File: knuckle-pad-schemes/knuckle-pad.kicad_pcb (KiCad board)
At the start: 2 copper layers, 127.6 x 115.3 mm, 67 parts, among them SW1 SW_Push, SW10 SW_Push, SW11 SW_Push, SW12 SW_Push, SW13 SW_Push, SW14 SW_Push, SW15 SW_Push, SW16 SW_Push, SW17 SW_Push, SW18 SW_Push, SW19 SW_Push, SW2 SW_Push, SW20 SW_Push, SW21 SW_Push, SW22 SW_Push, SW23 SW_Push, SW24 SW_Push, SW25 SW_Push, SW26 SW_Push, SW27 SW_Push, SW28 SW_Push, SW29 SW_Push, SW3 SW_Push, SW4 SW_Push, SW5 SW_Push, SW6 SW_Push, SW7 SW_Push, SW8 SW_Push, SW9 SW_Push, U1 ProMicro

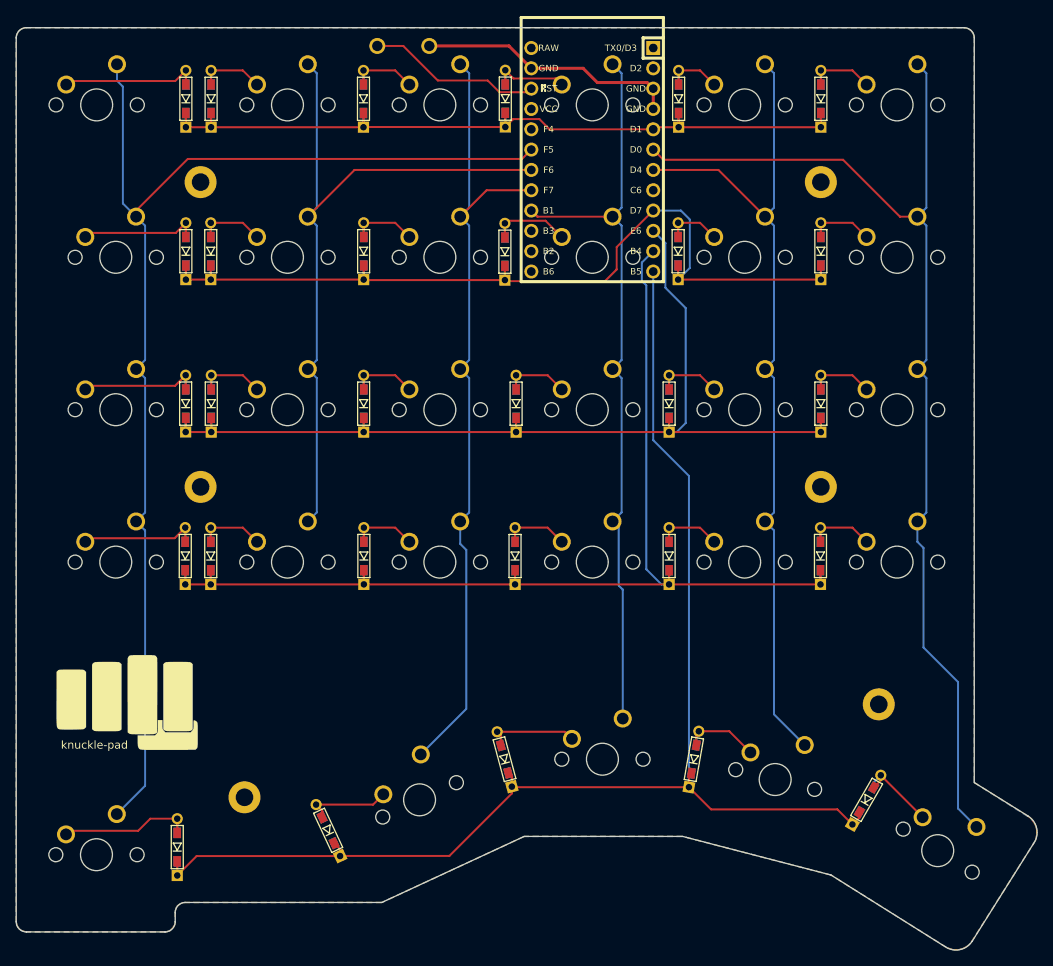
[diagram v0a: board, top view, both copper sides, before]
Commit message: clean up
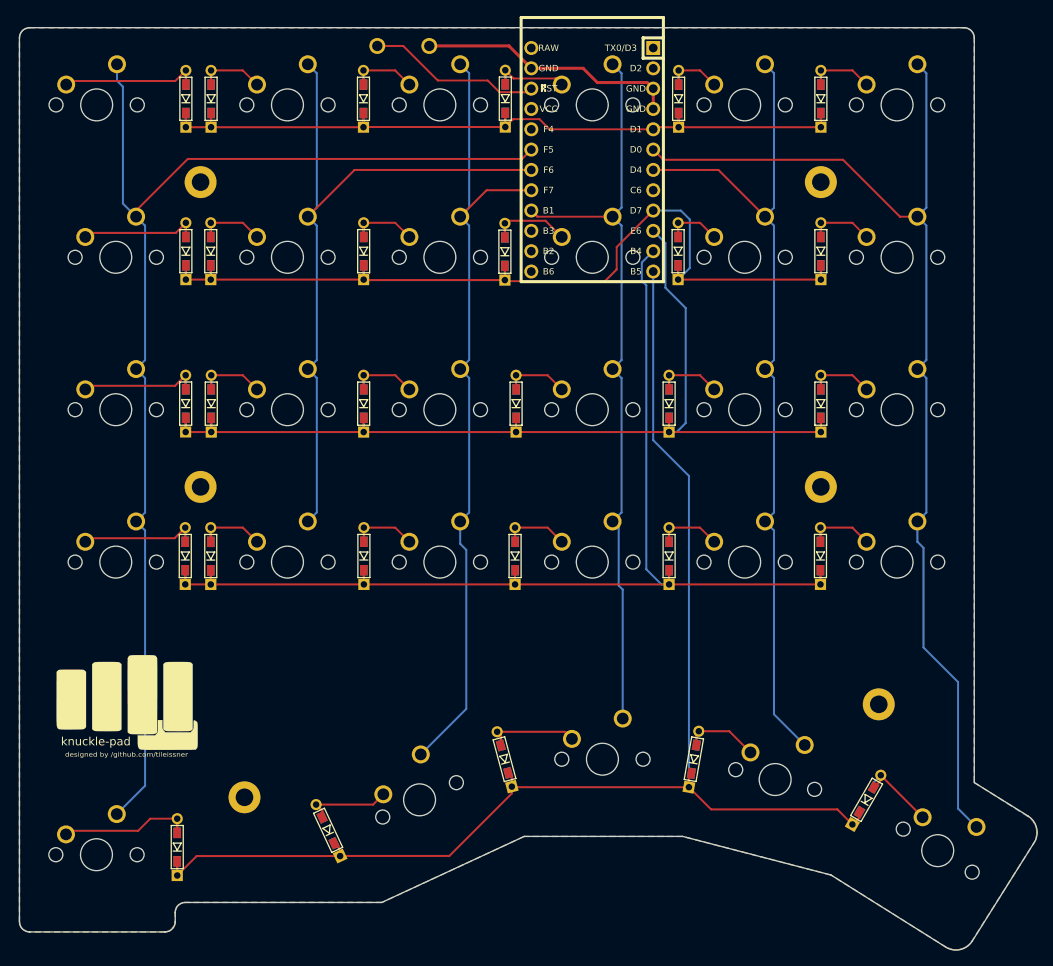
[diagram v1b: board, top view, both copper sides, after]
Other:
- board size 127.6 x 115.3 mm -> 127.2 x 115.3 mm
- board text added: "designed by /github.com/tileissner"
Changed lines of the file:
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@@
   (general
     (thickness 1.6)
-    (drawings 22)
+    (drawings 23)
     (tracks 372)
     (zones 0)
@@
     )
   )
-  (gr_text knuckle-pad (at 90.678 123.444) (layer F.SilkS)
-    (effects (font (size 1 1) (thickness 0.15)))
+  (gr_text "designed by /github.com/tileissner" (at 94.6912 124.64034) (layer F.SilkS)
+    (effects (font (size 0.5842 0.6477) (thickness 0.0762)))
+  )
+  (gr_arc (start 82.5754 35.052) (end 82.5754 33.782) (angle -90) (layer Edge.Cuts) (width 0.05))
+  (gr_arc (start 82.5754 145.542) (end 81.3054 145.542) (angle -90) (layer Edge.Cuts) (width 0.05))
+  (gr_text knuckle-pad (at 90.8558 123.00712) (layer F.SilkS)
+    (effects (font (size 1.0414 1.0414) (thickness 0.13335)))
   )
   (gr_arc (start 206.121001 134.365999) (end 207.391 132.334) (angle 93.53229458) (layer Edge.Cuts) (width 0.05))
   (gr_arc (start 198.374001 146.685001) (end 200.406 147.955) (angle 93.53229458) (layer Edge.Cuts) (width 0.05))
   (gr_line (start 200.66 35.052) (end 200.66 128.143) (layer Edge.Cuts) (width 0.05))
-  (gr_line (start 82.169 33.782) (end 199.39 33.782) (layer Edge.Cuts) (width 0.05))
-  (gr_line (start 80.899 145.542) (end 80.899 35.052) (layer Edge.Cuts) (width 0.05))
+  (gr_line (start 82.5754 33.782) (end 199.39 33.782) (layer Edge.Cuts) (width 0.05))
+  (gr_line (start 81.3054 145.542) (end 81.3054 35.052) (layer Edge.Cuts) (width 0.05))
   (gr_arc (start 199.39 35.052) (end 200.66 35.052) (angle -90) (layer Edge.Cuts) (width 0.05))
-  (gr_arc (start 82.169 35.052) (end 82.169 33.782) (angle -90) (layer Edge.Cuts) (width 0.05))
   (gr_line (start 102.0445 143.129) (end 116.713 143.129) (layer Edge.Cuts) (width 0.05))
   (gr_line (start 100.7745 145.542) (end 100.7745 144.399) (layer Edge.Cuts) (width 0.05))
-  (gr_line (start 82.169 146.812) (end 99.5045 146.812) (layer Edge.Cuts) (width 0.05))
+  (gr_line (start 82.5754 146.812) (end 99.5045 146.812) (layer Edge.Cuts) (width 0.05))
   (gr_arc (start 102.0445 144.399) (end 102.0445 143.129) (angle -90) (layer Edge.Cuts) (width 0.05))
   (gr_arc (start 99.5045 145.542) (end 99.5045 146.812) (angle -90) (layer Edge.Cuts) (width 0.05))
   (gr_line (start 116.713 143.129) (end 126.619 143.129) (layer Edge.Cuts) (width 0.05))
-  (gr_arc (start 82.169 145.542) (end 80.899 145.542) (angle -90) (layer Edge.Cuts) (width 0.05))
   (gr_line (start 207.391 132.334) (end 200.66 128.143) (layer Edge.Cuts) (width 0.05))
   (gr_line (start 126.619 143.129) (end 126.873 143.002) (layer Edge.Cuts) (width 0.05))
@@
         (xy 144.399 134.874) (xy 126.619 143.129) (xy 101.7905 143.129) (xy 101.346 143.3195) (xy 100.965 143.637)
         (xy 100.7745 144.2085) (xy 100.7745 145.6055) (xy 100.711 145.923) (xy 100.457 146.304) (xy 100.076 146.685)
-        (xy 99.568 146.812) (xy 82.169 146.812) (xy 81.661 146.685) (xy 81.28 146.431) (xy 81.026 146.05)
-        (xy 80.899 145.542) (xy 80.899 35.0012) (xy 80.9752 34.6456) (xy 81.2292 34.1884) (xy 81.5848 33.9344)
-        (xy 82.042 33.782) (xy 199.2884 33.782)
+        (xy 99.568 146.812) (xy 82.7278 146.812) (xy 82.3214 146.7866) (xy 81.7118 146.4818) (xy 81.4578 146.1516)
+        (xy 81.3054 145.542) (xy 81.3054 35.0266) (xy 81.3816 34.6456) (xy 81.6102 34.2138) (xy 81.8896 33.9852)
+        (xy 82.5246 33.782) (xy 199.2884 33.782)
       )
     )
@@
         (xy 126.619 143.129) (xy 101.7905 143.129) (xy 101.346 143.3195) (xy 100.965 143.637) (xy 100.7745 144.2085)
         (xy 100.7745 145.6055) (xy 100.711 145.923) (xy 100.457 146.304) (xy 100.076 146.685) (xy 99.568 146.812)
-        (xy 82.169 146.812) (xy 81.661 146.685) (xy 81.28 146.431) (xy 81.026 146.05) (xy 80.899 145.542)
-        (xy 80.899 35.0012) (xy 80.9752 34.6456) (xy 81.2292 34.1884) (xy 81.5848 33.9344) (xy 82.042 33.782)
+        (xy 82.7278 146.812) (xy 82.3214 146.7866) (xy 81.7118 146.4818) (xy 81.4578 146.1516) (xy 81.3054 145.53565)
+        (xy 81.3054 35.0266) (xy 81.3816 34.6456) (xy 81.6102 34.2138) (xy 81.8896 33.9852) (xy 82.5246 33.782)
         (xy 199.2884 33.782)
       )
